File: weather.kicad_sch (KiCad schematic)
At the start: 27 parts, among them J1 Conn_01x09_Socket, J2 BreakoutOfTemp+humid+pressure, Q1 2N7002H, Q2 2N7002H, U1 DRA818V, U2 TPS62132, U3 DS18B20, U4 DS18B20, U5 BMP280, U7 4554

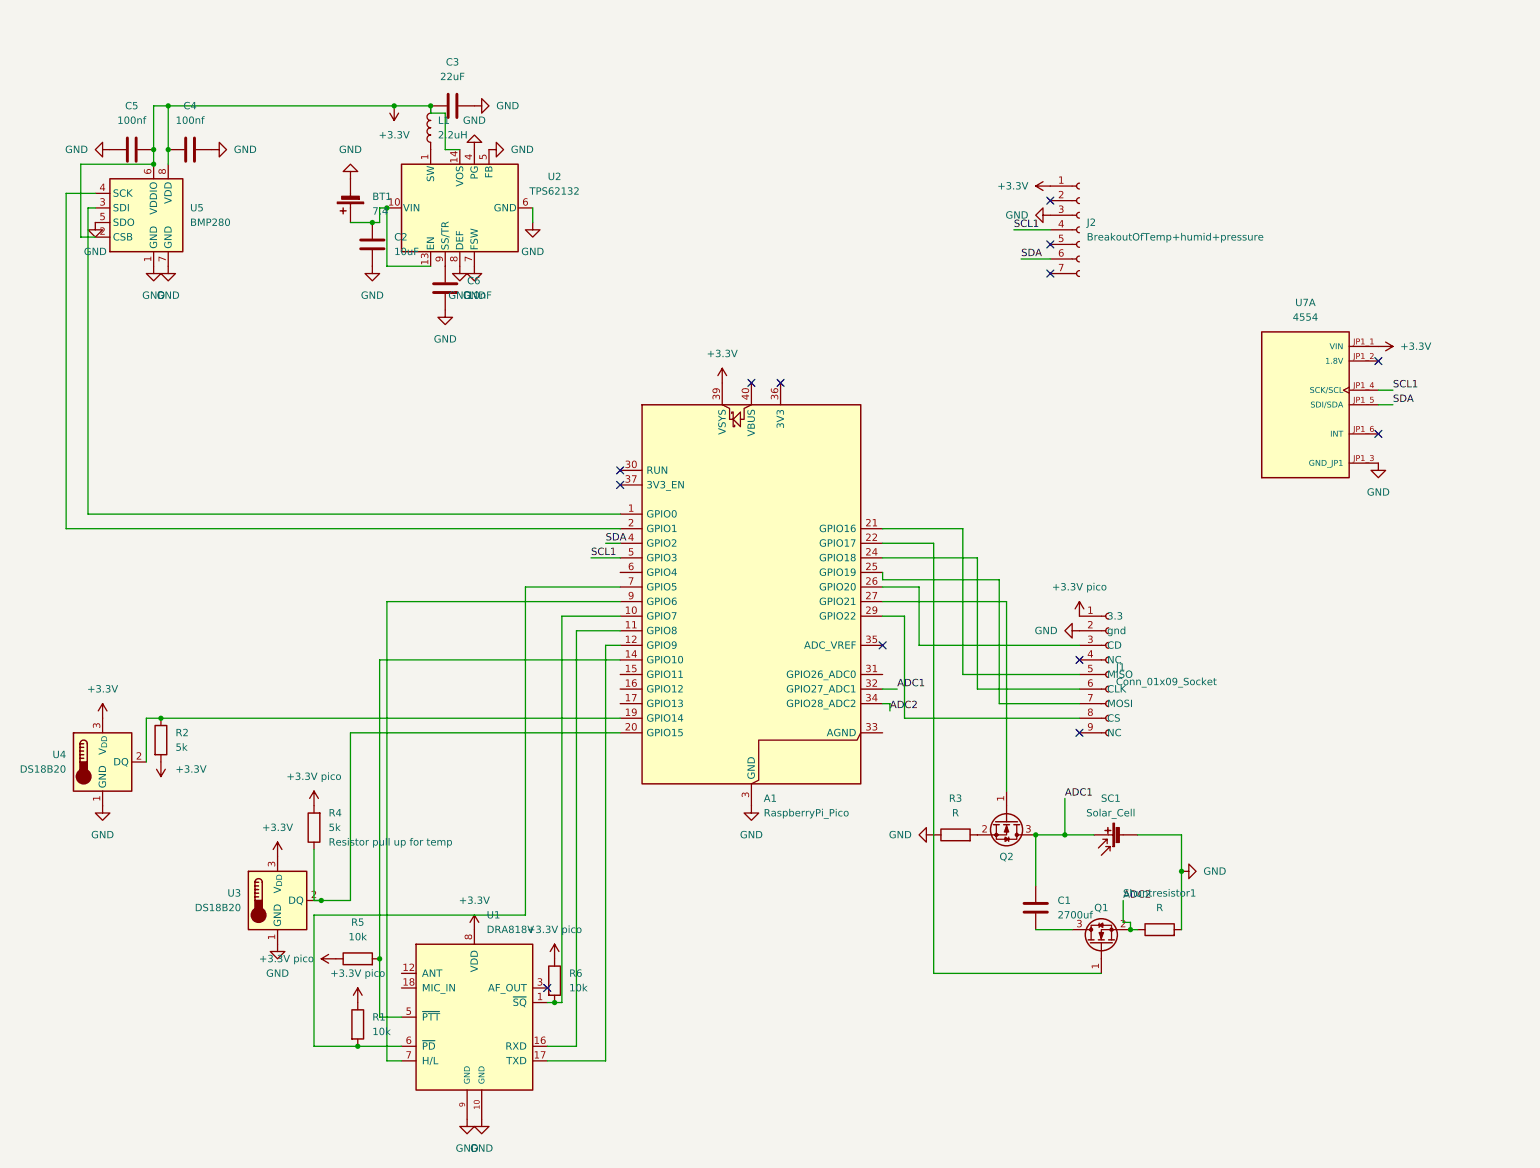
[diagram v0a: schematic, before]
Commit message: PCB layout preview
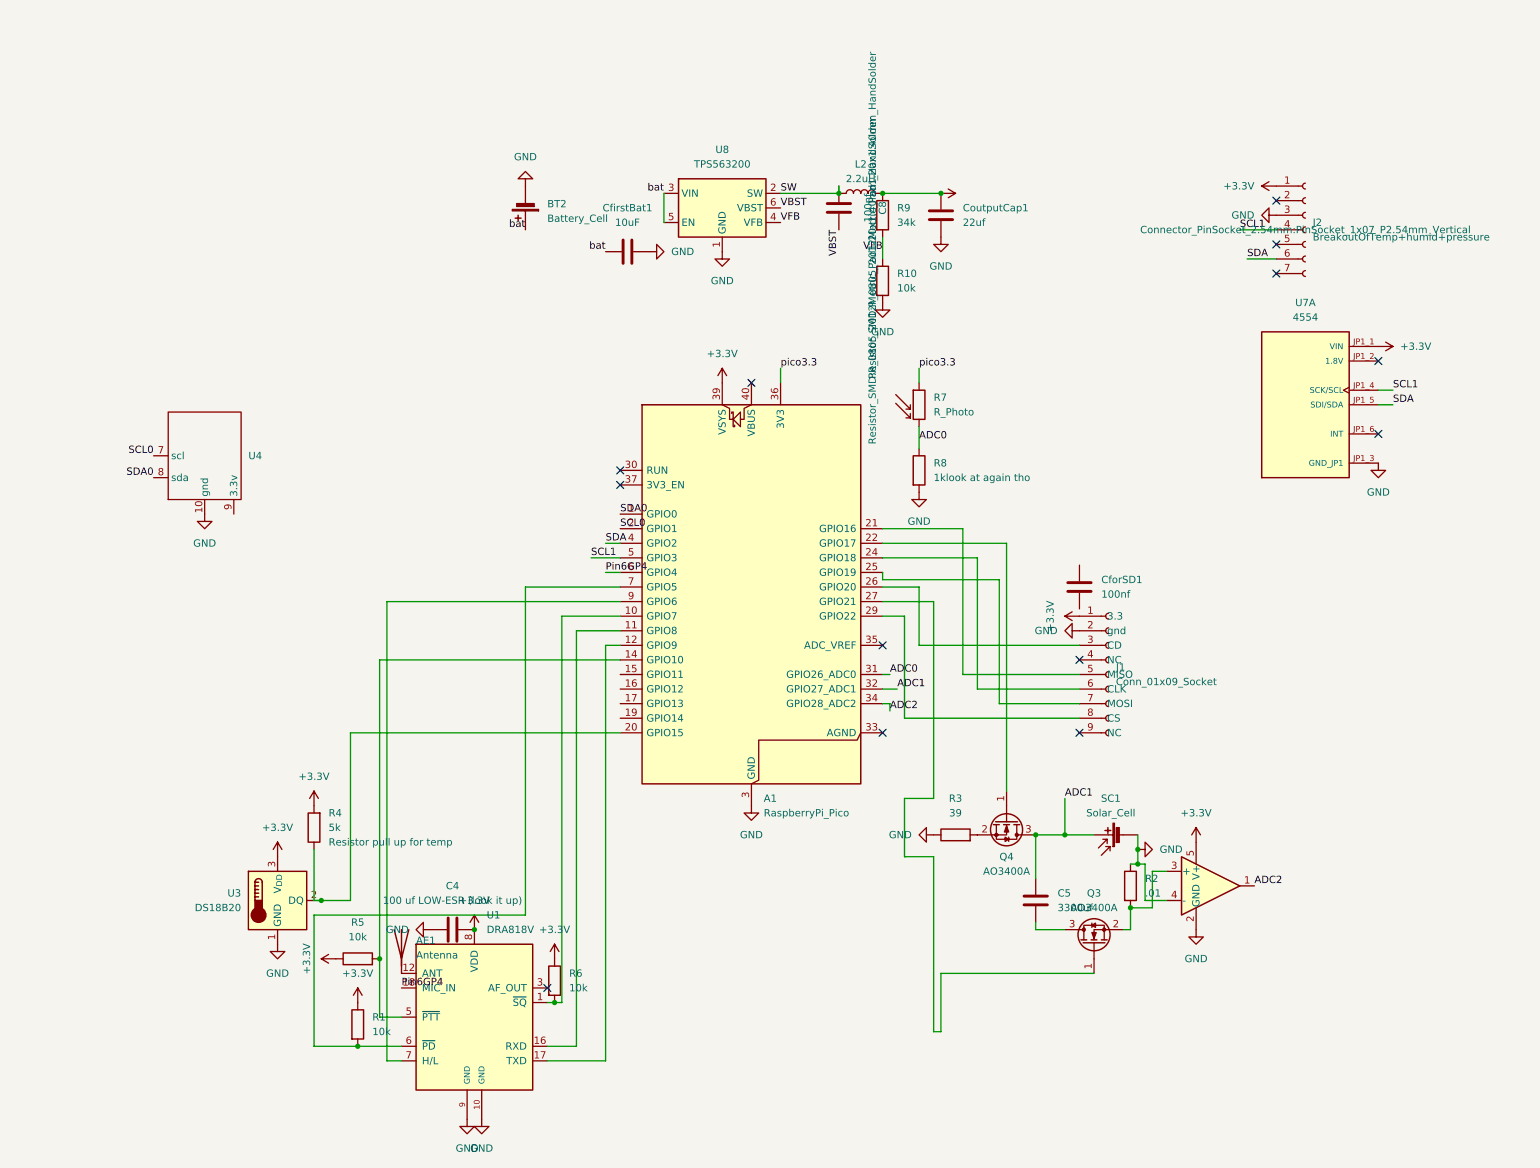
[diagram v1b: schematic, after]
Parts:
- removed BT1: 7.4, Connector_PinSocket_2.54mm:PinSocket_1x02_P2.54mm_Vertical, symbol Device:Battery_Cell
- removed C1: 2700uf, symbol Device:C
- removed C2: 10uF, symbol Device:C
- removed C3: 22uF, symbol Device:C
- removed C6: 10nF, symbol Device:C
- removed L1: 2.2uH, symbol Device:L
- removed Q1, Q2: 2N7002H, Package_TO_SOT_SMD:SOT-23, symbol Transistor_FET:2N7002H
- removed Shuntresistor1: R, symbol Device:R
- removed U2: TPS62132, Package_DFN_QFN:VQFN-16-1EP_3x3mm_P0.5mm_EP1.68x1.68mm_ThermalVias, symbol Regulator_Switching:TPS62132
- removed U4: DS18B20, Package_TO_SOT_THT:TO-92_Inline, symbol Sensor_Temperature:DS18B20
- removed U5: BMP280, Package_LGA:Bosch_LGA-8_2x2.5mm_P0.65mm_ClockwisePinNumbering, symbol Sensor_Pressure:BMP280
- added AE1: Antenna, symbol Device:Antenna
- added BT2: Battery_Cell, symbol Device:Battery_Cell
- added C8, CforSD1: 100nf, Capacitor_SMD:C_0805_2012Metric_Pad1.18x1.45mm_HandSolder, symbol Device:C
- added CfirstBat1: 10uF, Capacitor_SMD:C_0805_2012Metric_Pad1.18x1.45mm_HandSolder, symbol Device:C
- added CoutputCap1: 22uf, Capacitor_SMD:C_0805_2012Metric_Pad1.18x1.45mm_HandSolder, symbol Device:C
- added L2: 2.2uH, Inductor_SMD:L_0805_2012Metric_Pad1.05x1.20mm_HandSolder, symbol Device:L
- added Q3, Q4: AO3400A, Package_TO_SOT_SMD:SOT-23, symbol Transistor_FET:AO3400A
- added R10: 10k, Resistor_SMD:R_0805_2012Metric_Pad1.20x1.40mm_HandSolder, symbol Device:R
- added R7: R_Photo, symbol Device:R_Photo
- added R8: 1klook at again tho, Resistor_SMD:R_0805_2012Metric_Pad1.20x1.40mm_HandSolder, symbol Device:R
- added R9: 34k, Resistor_SMD:R_0805_2012Metric_Pad1.20x1.40mm_HandSolder, symbol Device:R
- added U4: (no value), PCM_SparkFun-GNSS:SparkFun GNSS Receiver Breakout - MAX-M10S (Qwiic), symbol PCM_SparkFun-GNSS:_1SparkFun_GNSS_Receiver_Breakout_-_MAX-M10S_(Qwiic)
- added U5: INA180A3, Package_TO_SOT_SMD:SOT-23-5, symbol Amplifier_Current:INA180A3
- added U8: TPS563200, Package_TO_SOT_SMD:SOT-23-6, symbol Regulator_Switching:TPS563200
- C4: value 100nf -> 100 uf LOW-ESR (look it up)
- C5: value 100nf -> 3300uf; footprint (none) -> Capacitor_THT:CP_Radial_D12.5mm_P5.00mm
- J2: footprint (none) -> Connector_PinSocket_2.54mm:PinSocket_1x07_P2.54mm_Vertical
- R1, R4, R5, R6: footprint (none) -> Resistor_SMD:R_0805_2012Metric_Pad1.20x1.40mm_HandSolder
- R2: value 5k -> .01; footprint (none) -> Resistor_SMD:R_0805_2012Metric_Pad1.20x1.40mm_HandSolder
- R3: value R -> 39; footprint (none) -> Resistor_SMD:R_0805_2012Metric_Pad1.20x1.40mm_HandSolder
- SC1: footprint Connector_PinSocket_2.54mm:PinSocket_1x02_P2.54mm_Vertical -> TestPoint:TestPoint_2Pads_Pitch5.08mm_Drill1.3mm
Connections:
- net +3.3V pico is gone; now on net +3.3V: J1.1 (3.3), R1.1, R4.2, R5.1, R6.1
- net +3.3V: now also C4.2, CoutputCap1.2, L2.2, R9.1, U5.5 (V+); no longer C4.1, C5.2, R2.2
- net ADC1: now also C5.1, Q4.3 (D)
- net ADC2: now also U5.1
- net GND: now also C4.1, R2.1, BT2.2 (-), CfirstBat1.2, CoutputCap1.1, R10.2, R8.2, U4.10 (gnd), U5.2 (GND), U5.4 (-), U8.1 (GND); no longer C4.2, C5.1
- net at R3.2: now also Q4.2 (S)
- net SDA0: now reaches A1.1 (GPIO0)
- net SDA0: now also U4.8 (sda)
- net SCL0: now reaches A1.2 (GPIO1)
- net SCL0: now also U4.7 (scl)
- net at A1.19 (GPIO14): no longer R2.1
- net at A1.22 (GPIO17): now also Q4.1 (G)
- net at U1.12 (ANT): now also AE1.1 (A)
- net Pin6GP4: now reaches U1.18 (MIC_IN)
- net Pin6GP4: now also A1.6 (GPIO4)
- net at A1.27 (GPIO21): now also Q3.1 (G)
- net ADC0: now reaches A1.31 (GPIO26_ADC0)
- net ADC0: now also R7.2, R8.1
- net pico3.3: now reaches A1.36 (3V3)
- net pico3.3: now also R7.1
- new net: Q3.2 (S), R2.2, U5.3 (+)
- new net: C5.2, Q3.3 (D)
- new net SW: C8.1, L2.1, U8.2 (SW)
- new net VBST: C8.2, U8.6 (VBST)
- new net VFB: R10.1, R9.2, U8.4 (VFB)
- new net bat: BT2.1 (+), CfirstBat1.1, U8.3 (VIN), U8.5 (EN)
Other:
- moved on the sheet: J2
